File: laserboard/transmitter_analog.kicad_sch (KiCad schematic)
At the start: 18 parts, among them Q1 AO3400A, Q3 AO3400A

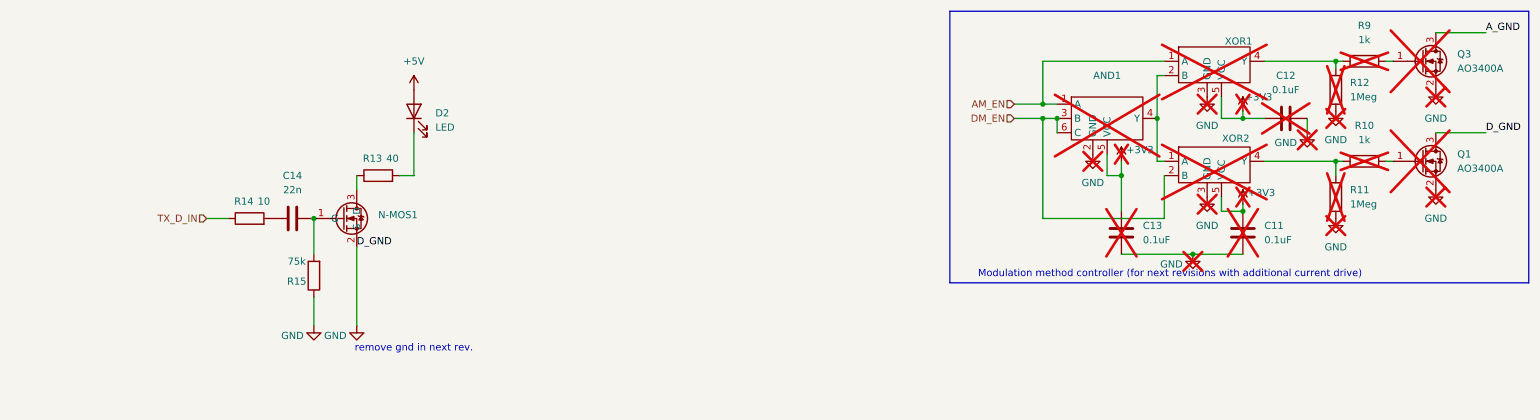
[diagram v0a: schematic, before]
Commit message: Backup
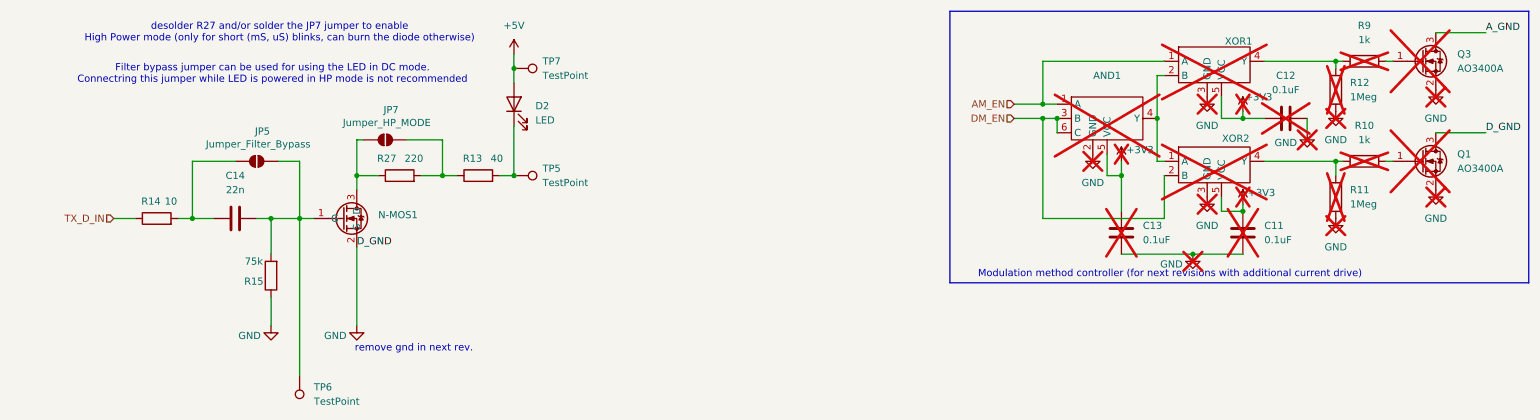
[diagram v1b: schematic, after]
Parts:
- added JP5: Jumper_Filter_Bypass, Jumper:SolderJumper-2_P1.3mm_Open_Pad1.0x1.5mm, symbol Jumper:SolderJumper_2_Open
- added JP7: Jumper_HP_MODE, Jumper:SolderJumper-2_P1.3mm_Open_Pad1.0x1.5mm, symbol Jumper:SolderJumper_2_Open
- added R27: 220, symbol Device:R
- added TP5, TP6, TP7: TestPoint, TestPoint:TestPoint_Pad_D2.0mm, symbol Connector:TestPoint
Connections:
- net +5V: now also TP7.1
- net at D2.1 (K), R13.2: now also TP5.1
- net at C14.1, R14.2: now also JP5.2 (B)
- net at C14.2, N-MOS1.1 (G), R15.2: now also JP5.1 (A), TP6.1
- net at N-MOS1.3 (D): now also JP7.2 (B), R27.1; no longer R13.1
- new net: JP7.1 (A), R13.1, R27.2
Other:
- note added: "Filter bypass jumper can be used for using the LED in DC mode. Connectring this jumper while LED is powered in HP mode is not recommended"
- note added: "desolder R27 and/or solder the JP7 jumper to enable High Power mode (only for short (mS, uS) blinks, can burn the diode otherwise)"
- moved on the sheet: C14, D2, R13, R14, R15

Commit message: Pre-PCB backup
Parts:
- C14: footprint (none) -> Capacitor_SMD:C_0402_1005Metric
- R13, R14, R15, R27: footprint (none) -> Resistor_SMD:R_0402_1005Metric
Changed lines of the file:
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@@
 			)
 		)
-		(property "Footprint" ""
+		(property "Footprint" "Resistor_SMD:R_0402_1005Metric"
 			(at 73.66 44.958 90)
 			(effects
@@
 			)
 		)
-		(property "Footprint" ""
+		(property "Footprint" "Capacitor_SMD:C_0402_1005Metric"
 			(at 48.26 49.8348 0)
 			(effects
@@
 			)
 		)
-		(property "Footprint" ""
+		(property "Footprint" "Resistor_SMD:R_0402_1005Metric"
 			(at 52.578 60.96 90)
 			(effects
@@
 			)
 		)
-		(property "Footprint" ""
+		(property "Footprint" "Resistor_SMD:R_0402_1005Metric"
 			(at 30.48 52.578 90)
 			(effects
@@
 			)
 		)
-		(property "Footprint" ""
+		(property "Footprint" "Resistor_SMD:R_0402_1005Metric"
 			(at 87.63 44.958 90)
 			(effects

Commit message: Post-production commit
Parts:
- C14: footprint Capacitor_SMD:C_0402_1005Metric -> parts:C_0402_1005Metric_nosilk
- R13, R14, R15, R27: footprint Resistor_SMD:R_0402_1005Metric -> parts:R_0402_1005Metric_nosilk
